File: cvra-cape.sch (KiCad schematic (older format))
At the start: 27 parts

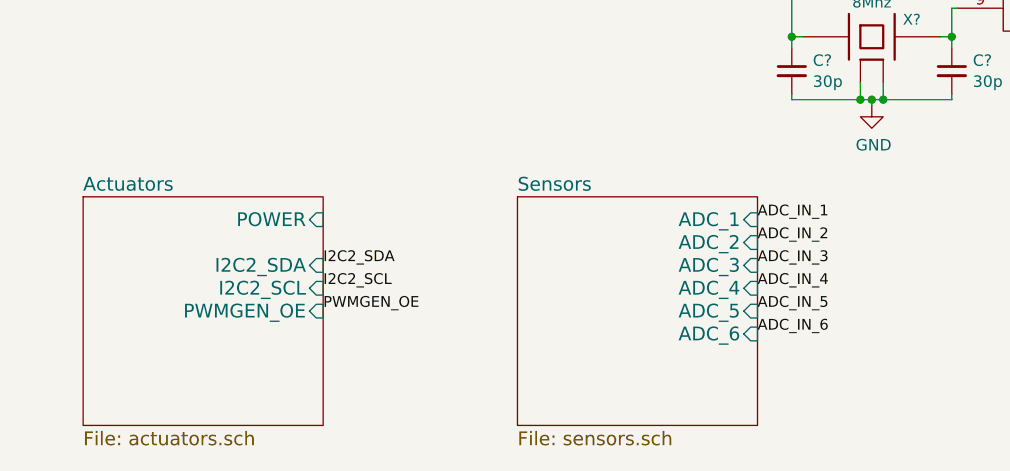
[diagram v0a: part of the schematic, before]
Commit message: Add RTC
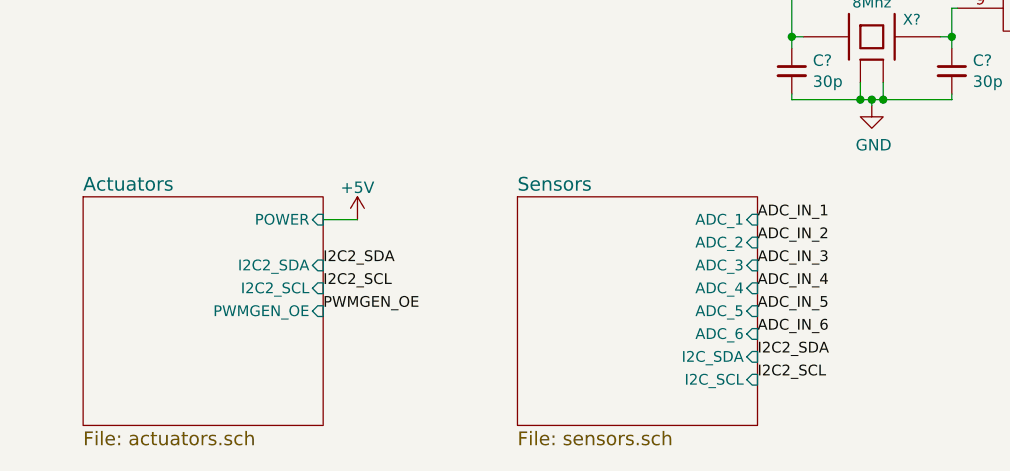
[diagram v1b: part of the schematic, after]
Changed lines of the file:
@@
 F0 "Actuators" 60
 F1 "actuators.sch" 60
-F2 "I2C2_SDA" I R 3850 6850 60
-F3 "I2C2_SCL" I R 3850 6950 60
-F4 "PWMGEN_OE" I R 3850 7050 60
-F5 "POWER" I R 3850 6650 60
+F2 "I2C2_SDA" I R 3850 6850 47
+F3 "I2C2_SCL" I R 3850 6950 47
+F4 "PWMGEN_OE" I R 3850 7050 47
+F5 "POWER" I R 3850 6650 47
 $EndSheet
 $Comp
@@
 F0 "Sensors" 60
 F1 "sensors.sch" 60
-F2 "ADC_1" I R 5750 6650 60
-F3 "ADC_2" I R 5750 6750 60
-F4 "ADC_3" I R 5750 6850 60
-F5 "ADC_4" I R 5750 6950 60
-F6 "ADC_5" I R 5750 7050 60
-F7 "ADC_6" I R 5750 7150 60
+F2 "ADC_1" I R 5750 6650 47
+F3 "ADC_2" I R 5750 6750 47
+F4 "ADC_3" I R 5750 6850 47
+F5 "ADC_4" I R 5750 6950 47
+F6 "ADC_5" I R 5750 7050 47
+F7 "ADC_6" I R 5750 7150 47
+F8 "I2C_SCL" I R 5750 7350 47
+F9 "I2C_SDA" I R 5750 7250 47
 $EndSheet
 Text Label 5750 6650 0    47   ~ 0
@@
 	1    0    0    -1
 $EndComp
+$Comp
+L +5V #PWR?
+U 1 1 56B4D7F8
+P 4000 6650
+F 0 "#PWR?" H 4000 6500 50  0001 C CNN
+F 1 "+5V" H 4000 6790 50  0000 C CNN
+F 2 "" H 4000 6650 60  0000 C CNN
+F 3 "" H 4000 6650 60  0000 C CNN
+	1    4000 6650
+	1    0    0    -1
+$EndComp
+Wire Wire Line
+	4000 6650 3850 6650
+Text Label 5750 7250 0    47   ~ 0
+I2C2_SDA
+Text Label 5750 7350 0    47   ~ 0
+I2C2_SCL
 $EndSCHEMATC
